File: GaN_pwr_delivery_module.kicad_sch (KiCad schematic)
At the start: 40 parts, among them J1 dcConn, J2 gateConn, J3 drainConn, Q1 AONS66920, U1 LDO40LPURY, U2 LM2662MX_NOPB, U3 LT4256-1CS8, U4 LM324

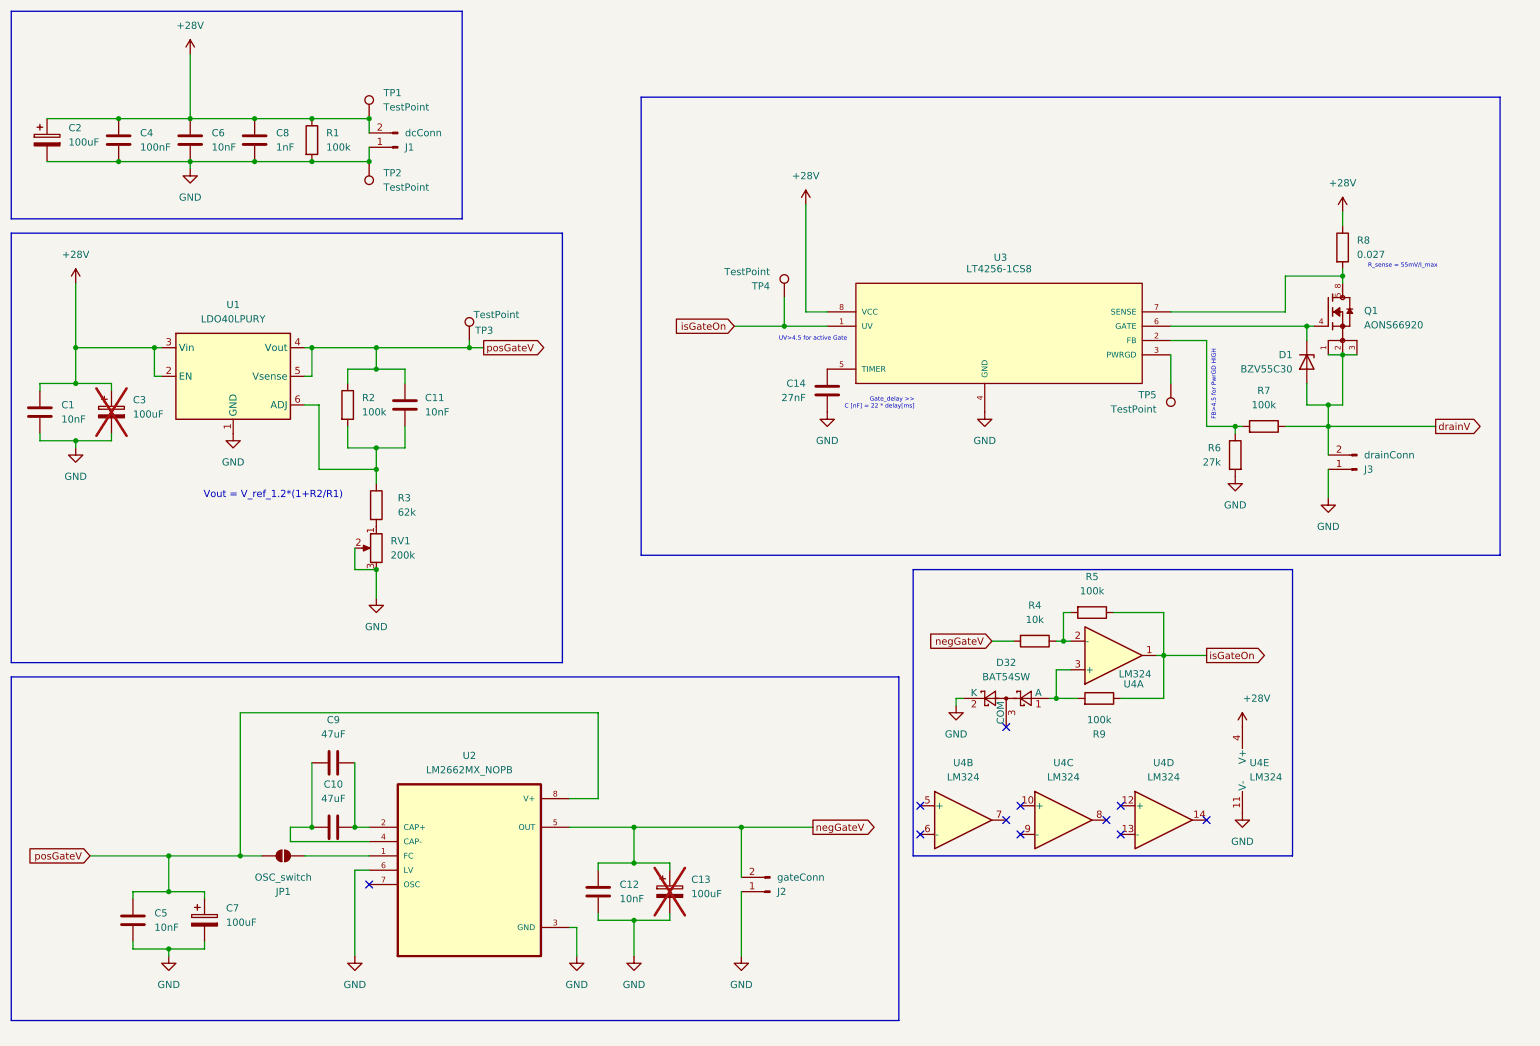
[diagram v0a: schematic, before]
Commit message: init ideas
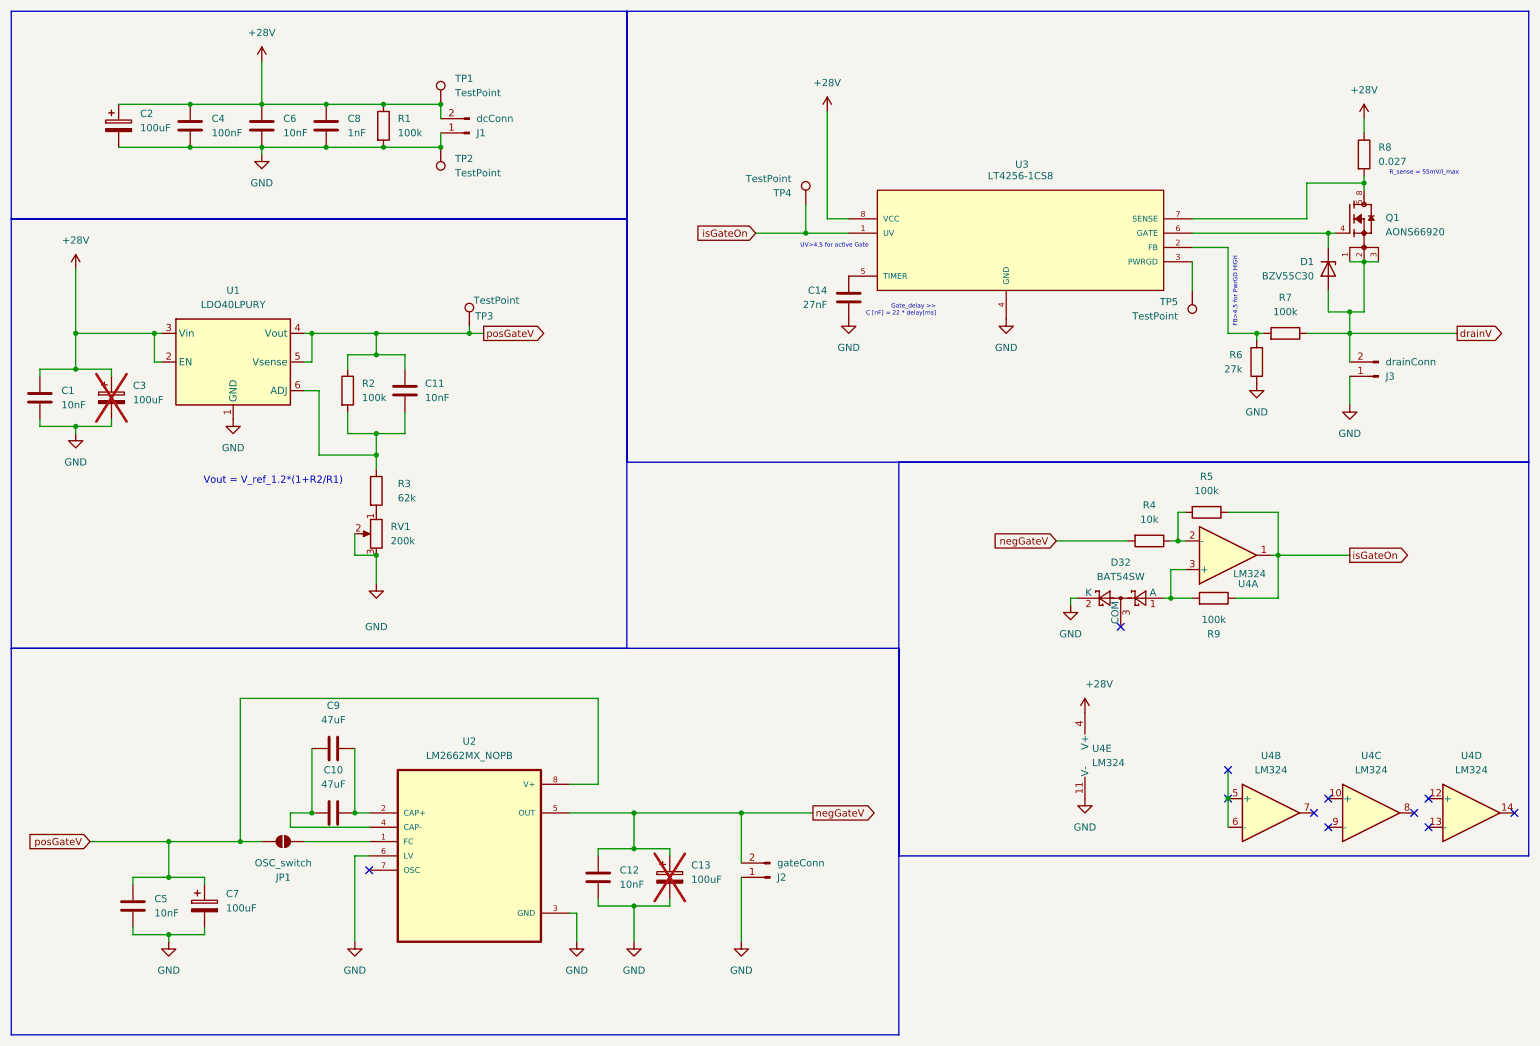
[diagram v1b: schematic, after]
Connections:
- net at U4.5 (+): now also U4.6 (-)
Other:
- moved on the sheet: C1, C10, C11, C12, C13, C14, C2, C3, C4, C5, C6, C7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
